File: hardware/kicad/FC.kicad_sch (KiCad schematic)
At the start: 6 parts, among them J1 xt30, U1 TPS7A4533DCQR

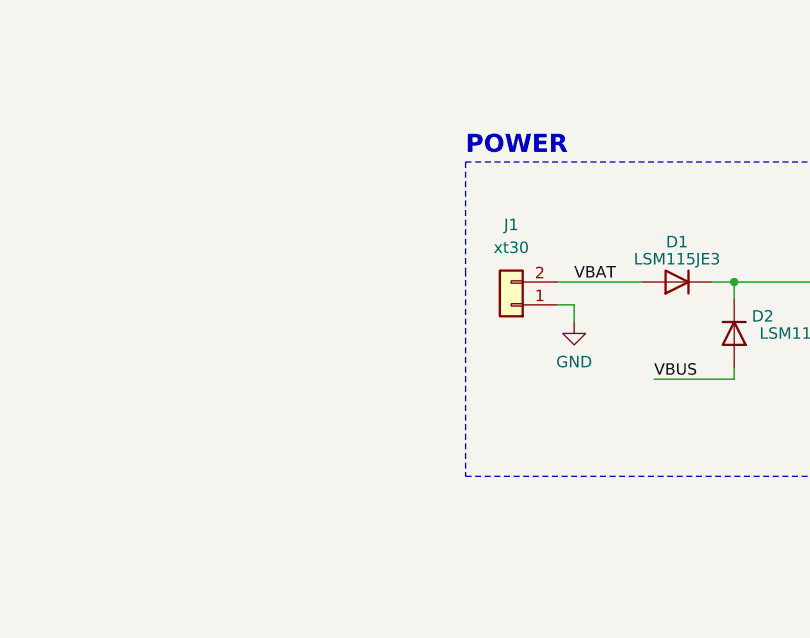
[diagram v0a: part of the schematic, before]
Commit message: ready for pcb
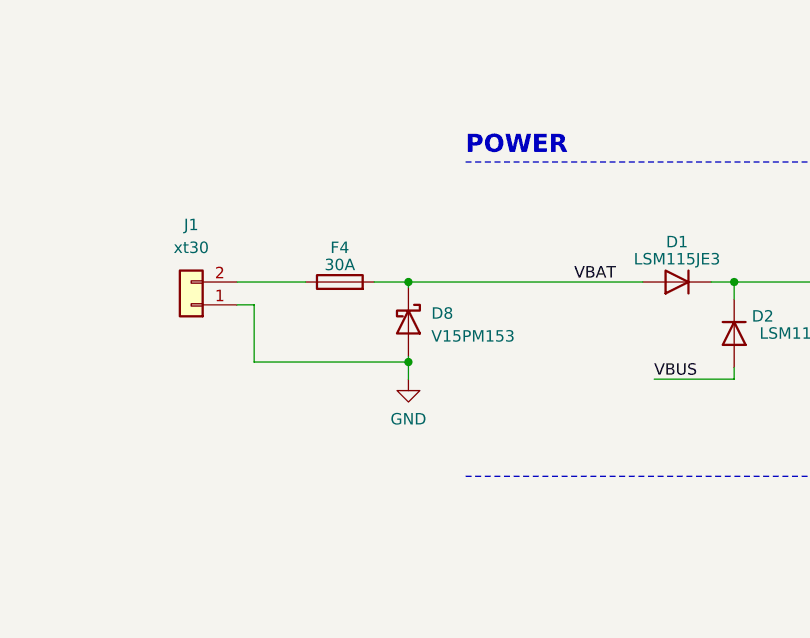
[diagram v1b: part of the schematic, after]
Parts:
- added D8: V15PM153, Package_TO_SOT_SMD:TO-277A, symbol Device:D_Schottky
- added F4: 30A, Resistor_SMD:R_1206_3216Metric, symbol Device:Fuse
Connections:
- net GND: now also D8.1 (A), D8.2 (A)
- net VBAT: now also D8.3 (K), F4.2; no longer J1.2 (N)
- new net: F4.1, J1.2 (N)
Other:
- moved on the sheet: J1
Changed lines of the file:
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@@
     (company "Missouri S&T Rocket Design Team")
   )
+  (junction (at 153.67 147.32) (diameter 0) (color 0 0 0 0)
+  )
   (junction (at 80.01 52.07) (diameter 0) (color 0 0 0 0)
+  )
+  (junction (at 153.67 156.21) (diameter 0) (color 0 0 0 0)
   )
   (junction (at 244.475 147.32) (diameter 0) (color 0 0 0 0)
@@
     (stroke (width 0) (type default))
   )
-  (wire (pts (xy 172.085 149.86) (xy 172.085 151.765))
-    (stroke (width 0) (type default))
-  )
   (wire (pts (xy 82.55 39.37) (xy 90.17 39.37))
     (stroke (width 0) (type default))
@@
     (stroke (width 0) (type default))
   )
+  (wire (pts (xy 134.62 147.32) (xy 142.24 147.32))
+    (stroke (width 0) (type default))
+  )
   (bus (pts (xy 154.94 52.07) (xy 192.405 52.07))
     (stroke (width 0) (type default))
@@
   )
   (wire (pts (xy 59.69 116.205) (xy 69.85 116.205))
+    (stroke (width 0) (type default))
+  )
+  (wire (pts (xy 136.525 156.21) (xy 153.67 156.21))
     (stroke (width 0) (type default))
   )
@@
     (stroke (width 0) (type default))
   )
-  (polyline (pts (xy 160.02 146.05) (xy 160.02 168.91))
-    (stroke (width 0) (type dash))
-  )
   (bus (pts (xy 15.24 180.34) (xy 15.24 184.15))
     (stroke (width 0) (type default))
   )
-  (wire (pts (xy 170.18 149.86) (xy 172.085 149.86))
+  (wire (pts (xy 153.67 156.21) (xy 153.67 158.115))
     (stroke (width 0) (type default))
   )
@@
     (stroke (width 0) (type dash))
   )
+  (wire (pts (xy 153.67 155.575) (xy 153.67 156.21))
+    (stroke (width 0) (type default))
+  )
   (wire (pts (xy 187.325 147.32) (xy 189.865 147.32))
     (stroke (width 0) (type default))
@@
     (stroke (width 0) (type dash))
   )
+  (wire (pts (xy 153.67 147.32) (xy 179.705 147.32))
+    (stroke (width 0) (type default))
+  )
   (bus (pts (xy 69.85 41.91) (xy 69.85 45.085))
     (stroke (width 0) (type default))
@@
   )
   (bus (pts (xy 229.87 41.91) (xy 229.87 45.085))
+    (stroke (width 0) (type default))
+  )
+  (wire (pts (xy 134.62 149.86) (xy 136.525 149.86))
     (stroke (width 0) (type default))
   )
@@
     (stroke (width 0) (type default))
   )
-  (polyline (pts (xy 160.02 133.985) (xy 160.02 146.05))
-    (stroke (width 0) (type dash))
-  )
   (wire (pts (xy 17.78 170.18) (xy 31.115 170.18))
     (stroke (width 0) (type default))
@@
     (stroke (width 0) (type default))
   )
+  (wire (pts (xy 153.67 147.32) (xy 153.67 147.955))
+    (stroke (width 0) (type default))
+  )
   (wire (pts (xy 59.69 123.825) (xy 69.85 123.825))
     (stroke (width 0) (type default))
@@
     (stroke (width 0) (type default))
   )
-  (wire (pts (xy 170.18 147.32) (xy 179.705 147.32))
+  (wire (pts (xy 149.86 147.32) (xy 153.67 147.32))
+    (stroke (width 0) (type default))
+  )
+  (wire (pts (xy 136.525 149.86) (xy 136.525 156.21))
     (stroke (width 0) (type default))
   )
@@
     )
   )
-  (symbol (lib_id "power:GND") (at 172.085 151.765 0) (unit 1)
+  (symbol (lib_id "power:GND") (at 153.67 158.115 0) (unit 1)
     (in_bom yes) (on_board yes) (dnp no) (fields_autoplaced)
-    (property "Reference" "#PWR01" (at 172.085 158.115 0)
-      (effects (font (size 1.27 1.27)) hide)
-    )
-    (property "Value" "GND" (at 172.085 156.21 0)
-      (effects (font (size 1.27 1.27)))
-    )
-    (property "Footprint" "" (at 172.085 151.765 0)
-      (effects (font (size 1.27 1.27)) hide)
-    )
-    (property "Datasheet" "" (at 172.085 151.765 0)
+    (property "Reference" "#PWR01" (at 153.67 164.465 0)
+      (effects (font (size 1.27 1.27)) hide)
+    )
+    (property "Value" "GND" (at 153.67 162.56 0)
+      (effects (font (size 1.27 1.27)))
+    )
+    (property "Footprint" "" (at 153.67 158.115 0)
+      (effects (font (size 1.27 1.27)) hide)
+    )
+    (property "Datasheet" "" (at 153.67 158.115 0)
       (effects (font (size 1.27 1.27)) hide)
     )
@@
     )
   )
-  (symbol (lib_id "Connector_Generic:Conn_01x02") (at 165.1 149.86 180) (unit 1)
+  (symbol (lib_id "Connector_Generic:Conn_01x02") (at 129.54 149.86 180) (unit 1)
     (in_bom yes) (on_board yes) (dnp no) (fields_autoplaced)
-    (property "Reference" "J1" (at 165.1 140.97 0)
-      (effects (font (size 1.27 1.27)))
-    )
-    (property "Value" "xt30" (at 165.1 143.51 0)
-      (effects (font (size 1.27 1.27)))
-    )
-    (property "Footprint" "XT30PW-M:AMASS_XT30PW-M" (at 162.56 139.7 0)
-      (effects (font (size 1.27 1.27)) hide)
-    )
-    (property "Datasheet" "~" (at 165.1 149.86 0)
-      (effects (font (size 1.27 1.27)) hide)
-    )
-    (property "Amazon" "https://www.amazon.com/Amass-XT30PW-Upgrade-Connectors-Battery/dp/B099F2PXYN#customerReviews" (at 162.56 139.7 0)
+    (property "Reference" "J1" (at 129.54 140.97 0)
+      (effects (font (size 1.27 1.27)))
+    )
+    (property "Value" "xt30" (at 129.54 143.51 0)
+      (effects (font (size 1.27 1.27)))
+    )
+    (property "Footprint" "XT30PW-M:AMASS_XT30PW-M" (at 127 139.7 0)
+      (effects (font (size 1.27 1.27)) hide)
+    )
+    (property "Datasheet" "~" (at 129.54 149.86 0)
+      (effects (font (size 1.27 1.27)) hide)
+    )
+    (property "Amazon" "https://www.amazon.com/Amass-XT30PW-Upgrade-Connectors-Battery/dp/B099F2PXYN#customerReviews" (at 127 139.7 0)
       (effects (font (size 1.27 1.27)) hide)
     )
@@
     )
   )
+  (symbol (lib_id "Device:D_Schottky") (at 153.67 151.765 270) (unit 1)
+    (in_bom yes) (on_board yes) (dnp no) (fields_autoplaced)
+    (property "Reference" "D8" (at 156.21 150.8125 90)
+      (effects (font (size 1.27 1.27)) (justify left))
+    )
+    (property "Value" "V15PM153" (at 156.21 153.3525 90)
+      (effects (font (size 1.27 1.27)) (justify left))
+    )
+    (property "Footprint" "Package_TO_SOT_SMD:TO-277A" (at 163.83 154.305 0)
+      (effects (font (size 1.27 1.27)) hide)
+    )
+    (property "Datasheet" "https://www.vishay.com/docs/87206/v15pm153.pdf" (at 163.83 154.305 0)
+      (effects (font (size 1.27 1.27)) hide)
+    )
+    (property "Digikey" "https://www.digikey.com/en/products/detail/vishay-general-semiconductor-diodes-division/V15PM153-M3-I/16683129" (at 163.83 154.305 0)
+      (effects (font (size 1.27 1.27)) hide)
+    )
+    (pin "3")
+    (pin "2")
+    (pin "1")
+    (instances
+      (project "FC"
+        (path "/54cce219-8b98-4e71-96c4-f9ee784aa3bc"
+          (reference "D8") (unit 1)
+        )
+      )
+    )
+  )
   (symbol (lib_id "Device:D") (at 183.515 147.32 180) (unit 1)
     (in_bom yes) (on_board yes) (dnp no)
@@
         )
       )
+    )
+  )
+  (symbol (lib_id "Device:Fuse") (at 146.05 147.32 90) (unit 1)
+    (in_bom yes) (on_board yes) (dnp no)
+    (property "Reference" "F4" (at 146.05 143.51 90)
+      (effects (font (size 1.27 1.27)))
+    )
+    (property "Value" "30A" (at 146.05 145.415 90)
+      (effects (font (size 1.27 1.27)))
+    )
+    (property "Footprint" "Resistor_SMD:R_1206_3216Metric" (at 146.05 149.098 90)
+      (effects (font (size 1.27 1.27)) hide)
+    )
+    (property "Datasheet" "https://www.belfuse.com/resources/datasheets/circuitprotection/ds-cp-c1h-series.pdf" (at 146.05 147.32 0)
+      (effects (font (size 1.27 1.27)) hide)
+    )
+    (property "Digikey" "https://www.digikey.com/en/products/detail/bel-fuse-inc/0685H9300-01/5466710?s=N4IgTCBcDaIAwDYAcBWAEgTgMxziAugL5A" (at 146.05 147.32 0)
+      (effects (font (size 1.27 1.27)) hide)
+    )
+    (pin "1")
+    (pin "2")
+    (instances
+      (project "FC"
+        (path "/54cce219-8b98-4e71-96c4-f9ee784aa3bc/047c0ef5-e762-41a7-bfd7-fdc982a27304"
+          (reference "F4") (unit 1)
+        )
+        (path "/54cce219-8b98-4e71-96c4-f9ee784aa3bc"
+          (reference "F2") (unit 1)
+        )
+      )

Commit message: sync
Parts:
- J1: footprint XT30PW-M:AMASS_XT30PW-M -> Connector_AMASS:AMASS_XT30PW-M_1x02_P2.50mm_Horizontal
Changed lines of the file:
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@@
       (effects (font (size 1.27 1.27)))
     )
-    (property "Footprint" "XT30PW-M:AMASS_XT30PW-M" (at 127 139.7 0)
+    (property "Footprint" "Connector_AMASS:AMASS_XT30PW-M_1x02_P2.50mm_Horizontal" (at 127 139.7 0)
       (effects (font (size 1.27 1.27)) hide)
     )
